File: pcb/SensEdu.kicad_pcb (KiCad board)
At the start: 4 copper layers, 99.1 x 54 mm, 147 parts, among them J1 Power, J10 Barrel_Jack_Switch, J11 Conn_01x04_Pin, J12 Conn_01x04_Pin, J13 Conn_02x01, J14 Conn_02x01, J15 Conn_02x01, J16 Conn_02x01, J17 Conn_03x01, J18 Conn_03x01, J19 Conn_03x01, J2 PWM, J20 Conn_01x04_Pin, J3 Analog, J4 PWM, J5 Analog, J6 Communication, J7 Digital, J8 Conn_03x01, J9 Conn_01x04_Pin, U1 AD8426ACPZ-R7, U12 TLS850C2TE_V33, U13 NCP1117-2.5_SOT223, U2 AD8426ACPZ-R7, U3 LT1790ACS6-1.25, U4 R_8_ADI, U5 AD8426ACPZ-R7, U6 AD8426ACPZ-R7, U7 R_8_ADI, U8 DPS310XTSA1

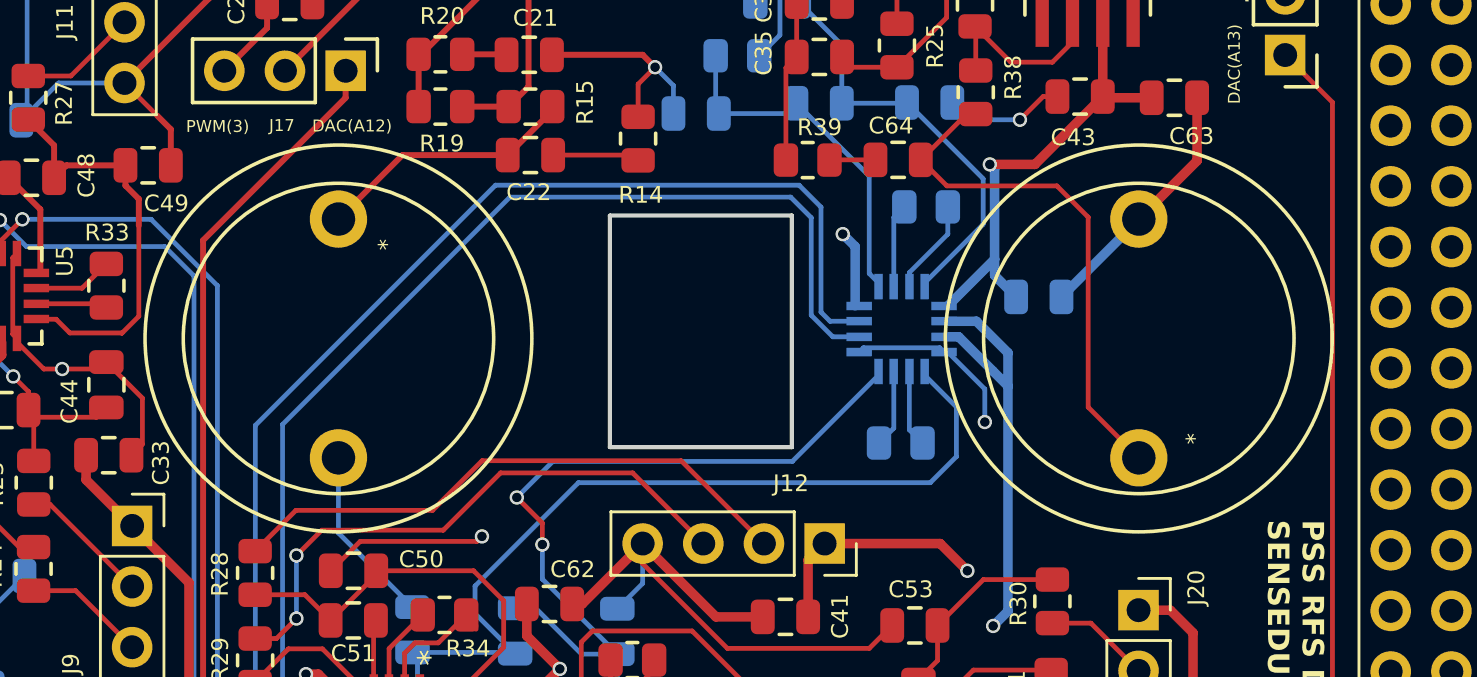
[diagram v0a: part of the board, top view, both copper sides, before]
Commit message: updates
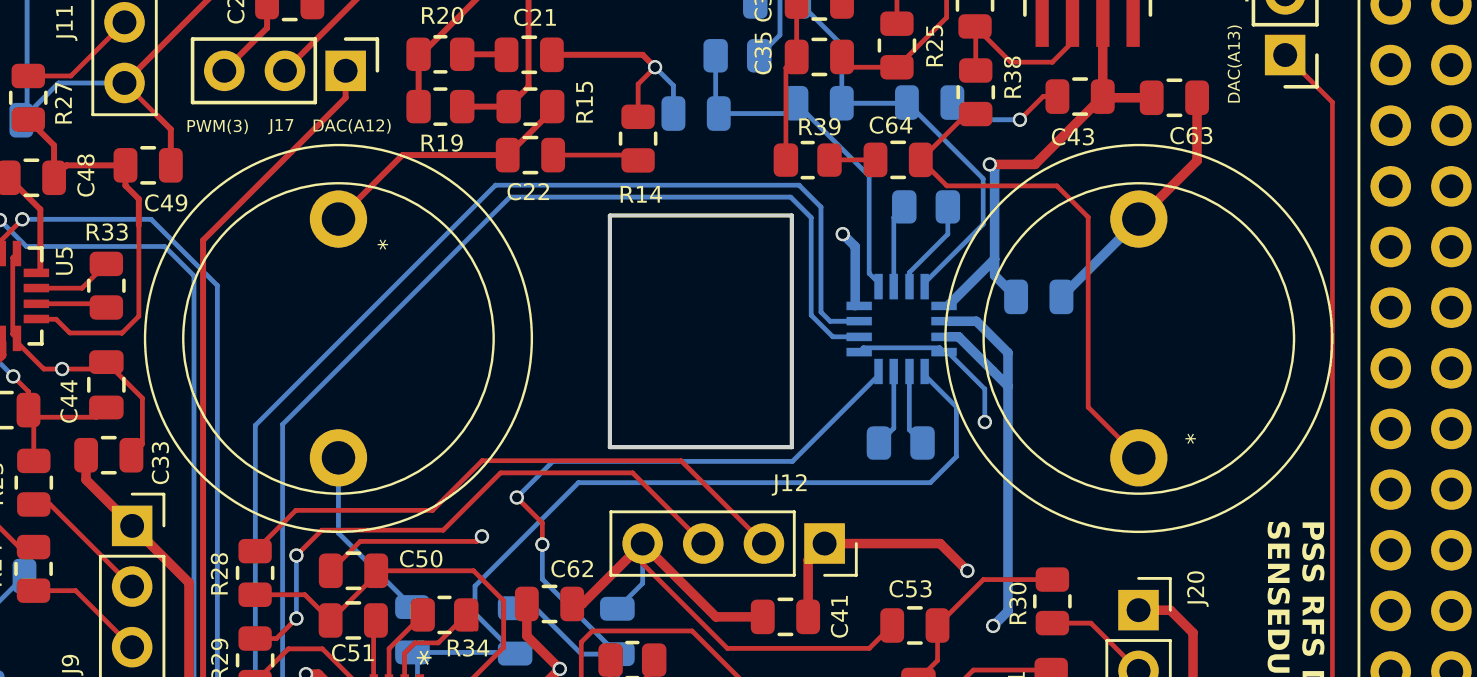
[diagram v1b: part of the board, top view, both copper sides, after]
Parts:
- LS1, LS2: footprint Speaker:328ST16M_Speaker -> SensEdu:328ST16M_Speaker
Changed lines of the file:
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@@
 		)
 	)
-	(footprint "Speaker:328ST16M_Speaker"
+	(footprint "SensEdu:328ST16M_Speaker"
 		(layer "F.Cu")
 		(at 183.43 73.35 90)
@@
 		(property "Reference" "LS2"
 			(at 0 -2.92 90)
-			(unlocked yes)
 			(layer "F.SilkS")
 			(hide yes)
 			(effects
 				(font
-					(size 0.7 0.7)
+					(size 1 1)
 					(thickness 0.15)
 				)
@@
 		(property "Value" "Speaker_Ultrasound"
 			(at 0 2.92 90)
-			(unlocked yes)
 			(layer "F.Fab")
 			(effects
@@
 			)
 		)
-		(property "Description" "Ultrasonic transducer"
+		(property "Description" ""
 			(at 0 0 90)
 			(layer "F.Fab")
@@
 			(end 8.1 0)
 			(stroke
-				(width 0.15)
+				(width 0.1)
 				(type default)
 			)
@@
 			(end 6.5 0)
 			(stroke
-				(width 0.15)
+				(width 0.1)
 				(type default)
 			)
@@
 		)
 		(embedded_fonts no)
-		(model "${KICAD6_3DMODEL_DIR}/Resistor_THT.3dshapes/R_Axial_DIN0411_L9.9mm_D3.6mm_P12.70mm_Horizontal.wrl"
+		(model "${KIPRJMOD}/libraries/3D/328ST16M.stp"
 			(offset
 				(xyz 0 0 0)
@@
 		)
 	)
-	(footprint "Speaker:328ST16M_Speaker"
+	(footprint "SensEdu:328ST16M_Speaker"
 		(layer "F.Cu")
 		(at 149.91 73.35 -90)
@@
 		(tags "328ST16M_Speaker")
 		(property "Reference" "LS1"
-			(at 0 -2.92 90)
-			(unlocked yes)
+			(at 0 -2.92 270)
 			(layer "F.SilkS")
 			(hide yes)
 			(effects
 				(font
-					(size 0.7 0.7)
+					(size 1 1)
 					(thickness 0.15)
 				)
@@
 		)
 		(property "Value" "Speaker_Ultrasound"
-			(at 0 2.92 90)
-			(unlocked yes)
+			(at 0 2.92 270)
 			(layer "F.Fab")
 			(effects
@@
 		)
 		(property "Datasheet" ""
-			(at 0 0 90)
+			(at 0 0 270)
 			(layer "F.Fab")
 			(hide yes)
@@
 			)
 		)
-		(property "Description" "Ultrasonic transducer"
-			(at 0 0 90)
+		(property "Description" ""
+			(at 0 0 270)
 			(layer "F.Fab")
 			(hide yes)
@@
 			(end 6.5 0)
 			(stroke
-				(width 0.15)
+				(width 0.1)
 				(type default)
 			)
@@
 			(end 8.1 0)
 			(stroke
-				(width 0.15)
+				(width 0.1)
 				(type default)
 			)
@@
 		)
 		(embedded_fonts no)
-		(model "${KICAD6_3DMODEL_DIR}/Resistor_THT.3dshapes/R_Axial_DIN0411_L9.9mm_D3.6mm_P12.70mm_Horizontal.wrl"
+		(model "${KIPRJMOD}/libraries/3D/328ST16M.stp"
 			(offset
 				(xyz 0 0 0)
